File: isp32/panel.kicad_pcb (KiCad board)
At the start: 2 copper layers, 67 x 98 mm, 584 parts, among them J1 BAT1, J10 LoRa_ANT, J11 Power Modules, J12 Micro_SD_Card, J2 Switching, J3 USB_C_Receptacle_USB2.0, J4 ADC, J5 GPS_ANT, J6 F0, J7 F1, J8 BUZZ, J9 ANT, M1 Motor_Servo, M2 Motor_Servo, M3 Motor_Servo, M4 Motor_Servo, Q1 BSS138, Q2 S8050, Q3 IRLML6402, Q4 BSS138, Q5 IRLML6402, Q6 IRLML6402, Q8 BSS138, Q9 BSS138, SW1 RST, U1 AZ1117-3.3, U10 BMP280, U11 MPU-9250, U2 MP2315, U3 STM32G030F6, U4 AZ1117-1.8, U6 24LC32, U7 NEO-XM, U8 ESP32-S3-WROOM-1U, U9 RFM98W-315S2

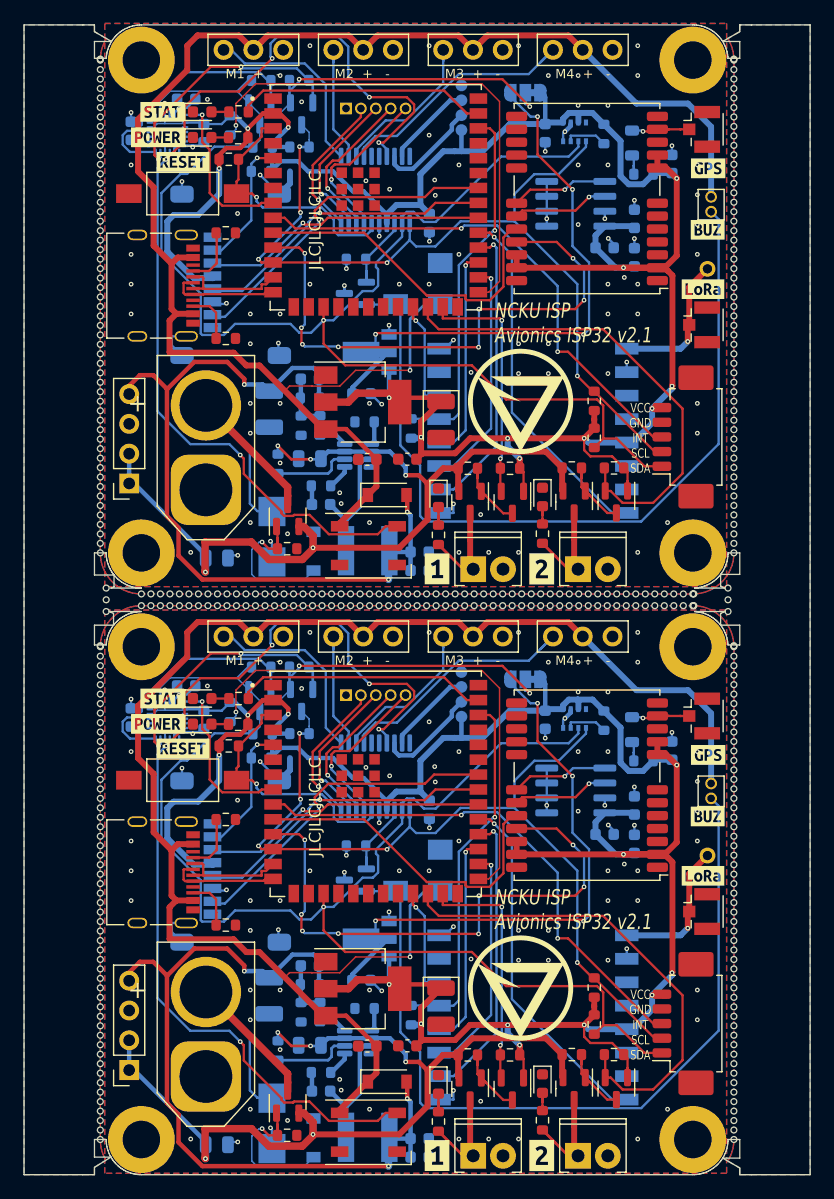
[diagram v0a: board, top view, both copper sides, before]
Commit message: chore: update isp32 project files
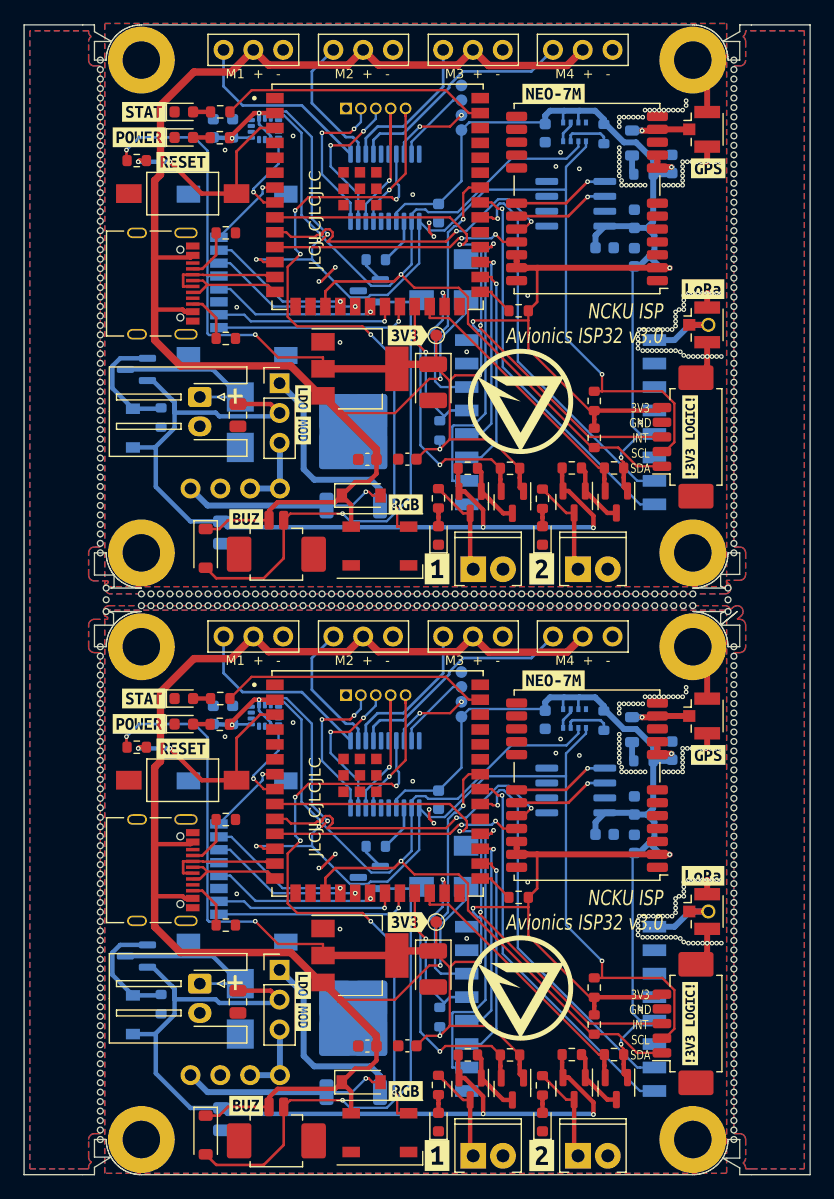
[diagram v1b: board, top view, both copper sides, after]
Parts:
- removed C1 (x2), C18 (x2), C8 (x2): 22u, Capacitor_SMD:C_0603_1608Metric
- removed the C12 at (107.0, 53.6)
- removed the C12 at (107.0, 103.6)
- removed the C15 at (87.9, 65.4)
- removed the C15 at (87.9, 115.4)
- removed C2 (x2): 220u, Capacitor_Tantalum_SMD:CP_EIA-3528-12_Kemet-T
- removed the C22 at (86.8, 29.2)
- removed the C22 at (86.8, 79.2)
- removed the C23 at (80.6, 79.0)
- removed the C23 at (80.6, 29.0)
- removed C24 (x2), C4 (x2): 100n, Capacitor_SMD:C_0603_1608Metric
- removed the C3 at (106.1, 86.9)
- removed the C3 at (106.1, 36.9)
- removed the C5 at (95.9, 107.0)
- removed the C5 at (95.9, 57.0)
- removed C7 (x2): NC, Capacitor_SMD:C_0603_1608Metric
- removed the D1 at (96.2, 114.9)
- removed the D1 at (96.2, 64.9)
- removed the D2 at (115.7, 110.2)
- removed the D2 at (115.7, 60.2)
- removed the D3 at (86.7, 77.4)
- removed the D3 at (86.7, 27.4)
- removed the D4 at (106.8, 60.3)
- removed the D4 at (106.8, 110.3)
- removed the D5 at (86.7, 29.6)
- removed the D5 at (86.7, 79.6)
- removed the D6 at (92.6, 113.6)
- removed the D6 at (92.6, 63.6)
- removed the D7 at (100.8, 114.4)
- removed the D7 at (100.8, 64.4)
- removed the D8 at (102.4, 110.1)
- removed the D8 at (102.4, 60.1)
- removed the J1 at (87.0, 109.6)
- removed the J1 at (87.0, 59.6)
- removed the J11 at (80.5, 59.1)
- removed the J11 at (80.5, 109.1)
- removed the J12 at (89.7, 91.3)
- removed the J12 at (89.7, 41.3)
- removed the J3 at (83.4, 42.2)
- removed the J3 at (83.4, 92.2)
- removed J8 (x2): BUZZ, Connector_PinHeader_1.27mm:PinHeader_1x02_P1.27mm_Vertical
- removed the J9 at (129.7, 90.8)
- removed the J9 at (129.7, 40.8)
- removed JP1 (x2): MPU VIO, Jumper:SolderJumper-3_P1.3mm_Bridged12_RoundedPad1.0x1.5mm_NumberLabels
- removed L3 (x2): 5.5, Inductor_SMD:L_Sunlord_SWPA5020S
- removed the LS1 at (105.1, 92.0)
- removed the LS1 at (105.1, 42.0)
- removed the Q2 at (99.7, 92.9)
- removed the Q2 at (99.7, 42.9)
- removed the Q6 at (94.0, 111.8)
- removed the Q6 at (94.0, 61.8)
- removed Q8 (x2), Q9 (x2): BSS138, Package_TO_SOT_SMD:SOT-23
- removed the R1 at (88.9, 31.5)
- removed the R1 at (88.9, 81.5)
- removed R10 (x2): 7k5, Resistor_SMD:R_0603_1608Metric
- removed R11 (x2): 40.2k, Resistor_SMD:R_0603_1608Metric
- removed R13 (x2), R17 (x2), R28 (x2), R29 (x2), R30 (x2), R33 (x2): 10k, Resistor_SMD:R_0603_1608Metric
- removed the R15 at (104.5, 54.4)
- removed the R15 at (104.5, 104.4)
- removed the R18 at (89.7, 29.6)
- removed the R18 at (89.7, 79.6)
- removed the R19 at (89.8, 77.4)
- removed the R19 at (89.8, 27.4)
- removed the R2 at (89.1, 28.6)
- removed the R2 at (89.1, 78.6)
- removed R21 (x2): 75k, Resistor_SMD:R_0603_1608Metric
- removed the R22 at (115.7, 113.4)
- removed the R22 at (115.7, 63.4)
- removed the R25 at (106.8, 63.5)
- removed the R25 at (106.8, 113.5)
- removed the R26 at (93.9, 64.6)
- removed the R26 at (93.9, 114.6)
- removed the R3 at (93.1, 57.4)
- removed the R3 at (93.1, 107.4)
- removed R8 (x2): 20, Resistor_SMD:R_0603_1608Metric
- removed R9 (x2): 20k, Resistor_SMD:R_0603_1608Metric
- removed REF** (x342): NPTH, NPTH
- removed the U1 at (100.4, 52.1)
- removed the U1 at (100.4, 102.1)
- removed U11 (x2): MPU-9250, Sensor_Motion:InvenSense_QFN-24_3x3mm_P0.4mm
- removed the U2 at (100.0, 106.7)
- removed the U2 at (100.0, 56.7)
- removed the U3 at (101.4, 84.1)
- removed the U3 at (101.4, 34.1)
- removed the U4 at (101.0, 47.9)
- removed the U4 at (101.0, 97.9)
- removed the U8 at (101.5, 34.7)
- removed the U8 at (101.5, 84.7)
- removed the U9 at (114.9, 54.6)
- removed the U9 at (114.9, 104.6)
- removed the kibuzzard-641A73E5 at (83.3, 27.4)
- removed the kibuzzard-641A73E5 at (83.3, 77.4)
- removed the kibuzzard-641A73FA at (82.9, 29.6)
- removed the kibuzzard-641A73FA at (82.9, 79.6)
- removed the kibuzzard-641A7704 at (129.8, 87.5)
- removed the kibuzzard-641A7704 at (129.8, 37.5)
- removed kibuzzard-642D96EE (x2): G***, kibuzzard-642D96EE
- removed kibuzzard-642D96F8 (x2): G***, kibuzzard-642D96F8
- removed the kibuzzard-642D97EE at (127.3, 104.1)
- removed the kibuzzard-642D97EE at (127.3, 54.1)
- added C12: 220u, Capacitor_Tantalum_SMD:CP_EIA-3528-12_Kemet-T, F.Cu at (106.4, 100.5)
- added C12: 220u, Capacitor_Tantalum_SMD:CP_EIA-3528-12_Kemet-T, F.Cu at (106.4, 50.5)
- added C15: 10u, Capacitor_SMD:C_0805_2012Metric, B.Cu at (88.3, 113.3)
- added C15: 10u, Capacitor_SMD:C_0805_2012Metric, B.Cu at (88.3, 63.3)
- added C22: 1u, Capacitor_SMD:C_0603_1608Metric, B.Cu at (87.6, 78.8)
- added C22: 1u, Capacitor_SMD:C_0603_1608Metric, B.Cu at (87.6, 28.8)
- added C23: 100n, Capacitor_SMD:C_0603_1608Metric, B.Cu at (89.3, 28.8)
- added C23: 100n, Capacitor_SMD:C_0603_1608Metric, B.Cu at (89.3, 78.8)
- added C3: 100n, Capacitor_SMD:C_0603_1608Metric, B.Cu at (106.8, 86.0)
- added C3: 100n, Capacitor_SMD:C_0603_1608Metric, B.Cu at (106.8, 36.0)
- added C5: 100n, Capacitor_SMD:C_0805_2012Metric, F.Cu at (89.7, 53.3)
- added C5: 100n, Capacitor_SMD:C_0805_2012Metric, F.Cu at (89.7, 103.3)
- added D1: Zener, Diode_SMD:D_SOD-123, B.Cu at (80.8, 54.4)
- added D1: Zener, Diode_SMD:D_SOD-123, B.Cu at (80.8, 104.4)
- added D2: F0_LED, LED_SMD:LED_0603_1608Metric, F.Cu at (115.7, 63.5)
- added D2: F0_LED, LED_SMD:LED_0603_1608Metric, F.Cu at (115.7, 113.5)
- added D3: ESP_LED, LED_SMD:LED_0603_1608Metric, F.Cu at (85.1, 77.4)
- added D3: ESP_LED, LED_SMD:LED_0603_1608Metric, F.Cu at (85.1, 27.4)
- added D4: F1_LED, LED_SMD:LED_0603_1608Metric, F.Cu at (106.8, 113.5)
- added D4: F1_LED, LED_SMD:LED_0603_1608Metric, F.Cu at (106.8, 63.5)
- added D5: POWER, LED_SMD:LED_0603_1608Metric, F.Cu at (85.1, 29.6)
- added D5: POWER, LED_SMD:LED_0603_1608Metric, F.Cu at (85.1, 79.6)
- added D6: TVS, Diode_SMD:D_SMB, B.Cu at (89.9, 103.9)
- added D6: TVS, Diode_SMD:D_SMB, B.Cu at (89.9, 53.9)
- added D7: WS2812B, LED_SMD:LED_WS2812B_PLCC4_5.0x5.0mm_P3.2mm, F.Cu at (101.8, 64.4)
- added D7: WS2812B, LED_SMD:LED_WS2812B_PLCC4_5.0x5.0mm_P3.2mm, F.Cu at (101.8, 114.4)
- added D8: D_Shockley, Diode_SMD:D_SOD-123, F.Cu at (100.2, 60.1)
- added D8: D_Shockley, Diode_SMD:D_SOD-123, F.Cu at (100.2, 110.1)
- added D9: D_Small, Diode_SMD:D_SOD-123, F.Cu at (87.0, 64.6)
- added D9: D_Small, Diode_SMD:D_SOD-123, F.Cu at (87.0, 114.6)
- added J1: BAT1, Connector_JST:JST_XH_S2B-XH-A-1_1x02_P2.50mm_Horizontal, F.Cu at (86.5, 101.7)
- added J1: BAT1, Connector_JST:JST_XH_S2B-XH-A-1_1x02_P2.50mm_Horizontal, F.Cu at (86.5, 51.7)
- added J11: Power Modules, Connector_PinSocket_2.54mm:PinSocket_1x04_P2.54mm_Vertical, B.Cu at (85.7, 59.5)
- added J11: Power Modules, Connector_PinSocket_2.54mm:PinSocket_1x04_P2.54mm_Vertical, B.Cu at (85.7, 109.5)
- added J12: Micro_SD_Card, Connector_Card:microSD_HC_Wuerth_693072010801, B.Cu at (89.7, 91.3)
- added J12: Micro_SD_Card, Connector_Card:microSD_HC_Wuerth_693072010801, B.Cu at (89.7, 41.3)
- added J13: VIN_SELECT, Connector_PinHeader_2.54mm:PinHeader_1x03_P2.54mm_Vertical, F.Cu at (93.3, 100.5)
- added J13: VIN_SELECT, Connector_PinHeader_2.54mm:PinHeader_1x03_P2.54mm_Vertical, F.Cu at (93.3, 50.5)
- added J14: BUZZ, Connector_Molex:Molex_PicoBlade_53261-0271_1x02-1MP_P1.25mm_Horizontal, F.Cu at (93.0, 64.6)
- added J14: BUZZ, Connector_Molex:Molex_PicoBlade_53261-0271_1x02-1MP_P1.25mm_Horizontal, F.Cu at (93.0, 114.6)
- added J3: USB_C_Receptacle_USB2.0, Connector_USB:USB_C_Receptacle_Palconn_UTC16-G, F.Cu at (83.4, 92.0)
- added J3: USB_C_Receptacle_USB2.0, Connector_USB:USB_C_Receptacle_Palconn_UTC16-G, F.Cu at (83.4, 42.0)
- added J9: ANT, Connector_PinHeader_2.00mm:PinHeader_1x01_P2.00mm_Vertical, B.Cu at (129.8, 95.6)
- added J9: ANT, Connector_PinHeader_2.00mm:PinHeader_1x01_P2.00mm_Vertical, B.Cu at (129.8, 45.6)
- added KiKit_MB_1_1: NPTH, NPTH, F.Cu at (78.0, 65.0)
- added KiKit_MB_1_10: NPTH, NPTH, F.Cu at (78.0, 57.7)
- added KiKit_MB_1_11: NPTH, NPTH, F.Cu at (78.0, 56.9)
- added KiKit_MB_1_12: NPTH, NPTH, F.Cu at (78.0, 56.1)
- added KiKit_MB_1_13: NPTH, NPTH, F.Cu at (78.0, 55.3)
- added KiKit_MB_1_14: NPTH, NPTH, F.Cu at (78.0, 54.5)
- added KiKit_MB_1_15: NPTH, NPTH, F.Cu at (78.0, 53.7)
- added KiKit_MB_1_16: NPTH, NPTH, F.Cu at (78.0, 52.9)
- added KiKit_MB_1_17: NPTH, NPTH, F.Cu at (78.0, 52.1)
- added KiKit_MB_1_18: NPTH, NPTH, F.Cu at (78.0, 51.3)
- added KiKit_MB_1_19: NPTH, NPTH, F.Cu at (78.0, 50.5)
- added KiKit_MB_1_2: NPTH, NPTH, F.Cu at (78.0, 64.2)
- added KiKit_MB_1_20: NPTH, NPTH, F.Cu at (78.0, 49.7)
- added KiKit_MB_1_21: NPTH, NPTH, F.Cu at (78.0, 48.8)
- added KiKit_MB_1_22: NPTH, NPTH, F.Cu at (78.0, 48.0)
- added KiKit_MB_1_23: NPTH, NPTH, F.Cu at (78.0, 47.2)
- added KiKit_MB_1_24: NPTH, NPTH, F.Cu at (78.0, 46.4)
- added KiKit_MB_1_25: NPTH, NPTH, F.Cu at (78.0, 45.6)
- added KiKit_MB_1_26: NPTH, NPTH, F.Cu at (78.0, 44.8)
- added KiKit_MB_1_27: NPTH, NPTH, F.Cu at (78.0, 44.0)
- added KiKit_MB_1_28: NPTH, NPTH, F.Cu at (78.0, 43.2)
- added KiKit_MB_1_29: NPTH, NPTH, F.Cu at (78.0, 42.4)
- added KiKit_MB_1_3: NPTH, NPTH, F.Cu at (78.0, 63.4)
- added KiKit_MB_1_30: NPTH, NPTH, F.Cu at (78.0, 41.6)
- added KiKit_MB_1_31: NPTH, NPTH, F.Cu at (78.0, 40.8)
- added KiKit_MB_1_32: NPTH, NPTH, F.Cu at (78.0, 40.0)
- added KiKit_MB_1_33: NPTH, NPTH, F.Cu at (78.0, 39.2)
- added KiKit_MB_1_34: NPTH, NPTH, F.Cu at (78.0, 38.3)
- added KiKit_MB_1_35: NPTH, NPTH, F.Cu at (78.0, 37.5)
- added KiKit_MB_1_36: NPTH, NPTH, F.Cu at (78.0, 36.7)
- added KiKit_MB_1_37: NPTH, NPTH, F.Cu at (78.0, 35.9)
- added KiKit_MB_1_38: NPTH, NPTH, F.Cu at (78.0, 35.1)
- added KiKit_MB_1_39: NPTH, NPTH, F.Cu at (78.0, 34.3)
- added KiKit_MB_1_4: NPTH, NPTH, F.Cu at (78.0, 62.6)
- added KiKit_MB_1_40: NPTH, NPTH, F.Cu at (78.0, 33.5)
- added KiKit_MB_1_41: NPTH, NPTH, F.Cu at (78.0, 32.7)
- added KiKit_MB_1_42: NPTH, NPTH, F.Cu at (78.0, 31.9)
- added KiKit_MB_1_43: NPTH, NPTH, F.Cu at (78.0, 31.1)
- added KiKit_MB_1_44: NPTH, NPTH, F.Cu at (78.0, 30.3)
- added KiKit_MB_1_45: NPTH, NPTH, F.Cu at (78.0, 29.5)
- added KiKit_MB_1_46: NPTH, NPTH, F.Cu at (78.0, 28.7)
- added KiKit_MB_1_47: NPTH, NPTH, F.Cu at (78.0, 27.8)
- added KiKit_MB_1_48: NPTH, NPTH, F.Cu at (78.0, 27.0)
- added KiKit_MB_1_49: NPTH, NPTH, F.Cu at (78.0, 26.2)
- added KiKit_MB_1_5: NPTH, NPTH, F.Cu at (78.0, 61.8)
- added KiKit_MB_1_50: NPTH, NPTH, F.Cu at (78.0, 25.4)
- added KiKit_MB_1_51: NPTH, NPTH, F.Cu at (78.0, 24.6)
- added KiKit_MB_1_52: NPTH, NPTH, F.Cu at (78.0, 23.8)
- added KiKit_MB_1_53: NPTH, NPTH, F.Cu at (78.0, 23.0)
- added KiKit_MB_1_6: NPTH, NPTH, F.Cu at (78.0, 61.0)
- added KiKit_MB_1_7: NPTH, NPTH, F.Cu at (78.0, 60.2)
- added KiKit_MB_1_8: NPTH, NPTH, F.Cu at (78.0, 59.3)
- added KiKit_MB_1_9: NPTH, NPTH, F.Cu at (78.0, 58.5)
- added KiKit_MB_2_1: NPTH, NPTH, F.Cu at (128.5, 68.5)
- added KiKit_MB_2_10: NPTH, NPTH, F.Cu at (121.2, 68.5)
- added KiKit_MB_2_11: NPTH, NPTH, F.Cu at (120.4, 68.5)
- added KiKit_MB_2_12: NPTH, NPTH, F.Cu at (119.6, 68.5)
- added KiKit_MB_2_13: NPTH, NPTH, F.Cu at (118.8, 68.5)
- added KiKit_MB_2_14: NPTH, NPTH, F.Cu at (118.0, 68.5)
- added KiKit_MB_2_15: NPTH, NPTH, F.Cu at (117.2, 68.5)
- added KiKit_MB_2_16: NPTH, NPTH, F.Cu at (116.3, 68.5)
- added KiKit_MB_2_17: NPTH, NPTH, F.Cu at (115.5, 68.5)
- added KiKit_MB_2_18: NPTH, NPTH, F.Cu at (114.7, 68.5)
- added KiKit_MB_2_19: NPTH, NPTH, F.Cu at (113.9, 68.5)
- added KiKit_MB_2_2: NPTH, NPTH, F.Cu at (127.7, 68.5)
- added KiKit_MB_2_20: NPTH, NPTH, F.Cu at (113.1, 68.5)
- added KiKit_MB_2_21: NPTH, NPTH, F.Cu at (112.3, 68.5)
- added KiKit_MB_2_22: NPTH, NPTH, F.Cu at (111.5, 68.5)
- added KiKit_MB_2_23: NPTH, NPTH, F.Cu at (110.7, 68.5)
- added KiKit_MB_2_24: NPTH, NPTH, F.Cu at (109.9, 68.5)
- added KiKit_MB_2_25: NPTH, NPTH, F.Cu at (109.1, 68.5)
- added KiKit_MB_2_26: NPTH, NPTH, F.Cu at (108.2, 68.5)
- added KiKit_MB_2_27: NPTH, NPTH, F.Cu at (107.4, 68.5)
- added KiKit_MB_2_28: NPTH, NPTH, F.Cu at (106.6, 68.5)
- added KiKit_MB_2_29: NPTH, NPTH, F.Cu at (105.8, 68.5)
- added KiKit_MB_2_3: NPTH, NPTH, F.Cu at (126.9, 68.5)
- added KiKit_MB_2_30: NPTH, NPTH, F.Cu at (105.0, 68.5)
- added KiKit_MB_2_31: NPTH, NPTH, F.Cu at (104.2, 68.5)
- added KiKit_MB_2_32: NPTH, NPTH, F.Cu at (103.4, 68.5)
- added KiKit_MB_2_33: NPTH, NPTH, F.Cu at (102.6, 68.5)
- added KiKit_MB_2_34: NPTH, NPTH, F.Cu at (101.8, 68.5)
- added KiKit_MB_2_35: NPTH, NPTH, F.Cu at (100.9, 68.5)
- added KiKit_MB_2_36: NPTH, NPTH, F.Cu at (100.1, 68.5)
- added KiKit_MB_2_37: NPTH, NPTH, F.Cu at (99.3, 68.5)
- added KiKit_MB_2_38: NPTH, NPTH, F.Cu at (98.5, 68.5)
- added KiKit_MB_2_39: NPTH, NPTH, F.Cu at (97.7, 68.5)
- added KiKit_MB_2_4: NPTH, NPTH, F.Cu at (126.1, 68.5)
- added KiKit_MB_2_40: NPTH, NPTH, F.Cu at (96.9, 68.5)
- added KiKit_MB_2_41: NPTH, NPTH, F.Cu at (96.1, 68.5)
- added KiKit_MB_2_42: NPTH, NPTH, F.Cu at (95.3, 68.5)
- added KiKit_MB_2_43: NPTH, NPTH, F.Cu at (94.5, 68.5)
- added KiKit_MB_2_44: NPTH, NPTH, F.Cu at (93.7, 68.5)
- added KiKit_MB_2_45: NPTH, NPTH, F.Cu at (92.8, 68.5)
- added KiKit_MB_2_46: NPTH, NPTH, F.Cu at (92.0, 68.5)
- added KiKit_MB_2_47: NPTH, NPTH, F.Cu at (91.2, 68.5)
- added KiKit_MB_2_48: NPTH, NPTH, F.Cu at (90.4, 68.5)
- added KiKit_MB_2_49: NPTH, NPTH, F.Cu at (89.6, 68.5)
- added KiKit_MB_2_5: NPTH, NPTH, F.Cu at (125.3, 68.5)
- added KiKit_MB_2_50: NPTH, NPTH, F.Cu at (88.8, 68.5)
- added KiKit_MB_2_51: NPTH, NPTH, F.Cu at (88.0, 68.5)
- added KiKit_MB_2_52: NPTH, NPTH, F.Cu at (87.2, 68.5)
- added KiKit_MB_2_53: NPTH, NPTH, F.Cu at (86.4, 68.5)
- added KiKit_MB_2_54: NPTH, NPTH, F.Cu at (85.6, 68.5)
- added KiKit_MB_2_55: NPTH, NPTH, F.Cu at (84.7, 68.5)
- added KiKit_MB_2_56: NPTH, NPTH, F.Cu at (83.9, 68.5)
- added KiKit_MB_2_57: NPTH, NPTH, F.Cu at (83.1, 68.5)
- added KiKit_MB_2_58: NPTH, NPTH, F.Cu at (82.3, 68.5)
- added KiKit_MB_2_59: NPTH, NPTH, F.Cu at (81.5, 68.5)
- added KiKit_MB_2_6: NPTH, NPTH, F.Cu at (124.4, 68.5)
- added KiKit_MB_2_7: NPTH, NPTH, F.Cu at (123.6, 68.5)
- added KiKit_MB_2_8: NPTH, NPTH, F.Cu at (122.8, 68.5)
- added KiKit_MB_2_9: NPTH, NPTH, F.Cu at (122.0, 68.5)
- added KiKit_MB_3_1: NPTH, NPTH, F.Cu at (132.0, 23.0)
- added KiKit_MB_3_10: NPTH, NPTH, F.Cu at (132.0, 30.3)
- added KiKit_MB_3_11: NPTH, NPTH, F.Cu at (132.0, 31.1)
- added KiKit_MB_3_12: NPTH, NPTH, F.Cu at (132.0, 31.9)
- added KiKit_MB_3_13: NPTH, NPTH, F.Cu at (132.0, 32.7)
- added KiKit_MB_3_14: NPTH, NPTH, F.Cu at (132.0, 33.5)
- added KiKit_MB_3_15: NPTH, NPTH, F.Cu at (132.0, 34.3)
- added KiKit_MB_3_16: NPTH, NPTH, F.Cu at (132.0, 35.1)
- added KiKit_MB_3_17: NPTH, NPTH, F.Cu at (132.0, 35.9)
- added KiKit_MB_3_18: NPTH, NPTH, F.Cu at (132.0, 36.7)
- added KiKit_MB_3_19: NPTH, NPTH, F.Cu at (132.0, 37.5)
- added KiKit_MB_3_2: NPTH, NPTH, F.Cu at (132.0, 23.8)
- added KiKit_MB_3_20: NPTH, NPTH, F.Cu at (132.0, 38.3)
- added KiKit_MB_3_21: NPTH, NPTH, F.Cu at (132.0, 39.2)
- added KiKit_MB_3_22: NPTH, NPTH, F.Cu at (132.0, 40.0)
- added KiKit_MB_3_23: NPTH, NPTH, F.Cu at (132.0, 40.8)
- added KiKit_MB_3_24: NPTH, NPTH, F.Cu at (132.0, 41.6)
- added KiKit_MB_3_25: NPTH, NPTH, F.Cu at (132.0, 42.4)
- added KiKit_MB_3_26: NPTH, NPTH, F.Cu at (132.0, 43.2)
- added KiKit_MB_3_27: NPTH, NPTH, F.Cu at (132.0, 44.0)
- added KiKit_MB_3_28: NPTH, NPTH, F.Cu at (132.0, 44.8)
- added KiKit_MB_3_29: NPTH, NPTH, F.Cu at (132.0, 45.6)
- added KiKit_MB_3_3: NPTH, NPTH, F.Cu at (132.0, 24.6)
- added KiKit_MB_3_30: NPTH, NPTH, F.Cu at (132.0, 46.4)
- added KiKit_MB_3_31: NPTH, NPTH, F.Cu at (132.0, 47.2)
- added KiKit_MB_3_32: NPTH, NPTH, F.Cu at (132.0, 48.0)
- added KiKit_MB_3_33: NPTH, NPTH, F.Cu at (132.0, 48.8)
- added KiKit_MB_3_34: NPTH, NPTH, F.Cu at (132.0, 49.7)
- added KiKit_MB_3_35: NPTH, NPTH, F.Cu at (132.0, 50.5)
- added KiKit_MB_3_36: NPTH, NPTH, F.Cu at (132.0, 51.3)
- added KiKit_MB_3_37: NPTH, NPTH, F.Cu at (132.0, 52.1)
- added KiKit_MB_3_38: NPTH, NPTH, F.Cu at (132.0, 52.9)
- added KiKit_MB_3_39: NPTH, NPTH, F.Cu at (132.0, 53.7)
- added KiKit_MB_3_4: NPTH, NPTH, F.Cu at (132.0, 25.4)
- added KiKit_MB_3_40: NPTH, NPTH, F.Cu at (132.0, 54.5)
- added KiKit_MB_3_41: NPTH, NPTH, F.Cu at (132.0, 55.3)
- added KiKit_MB_3_42: NPTH, NPTH, F.Cu at (132.0, 56.1)
- added KiKit_MB_3_43: NPTH, NPTH, F.Cu at (132.0, 56.9)
- added KiKit_MB_3_44: NPTH, NPTH, F.Cu at (132.0, 57.7)
- added KiKit_MB_3_45: NPTH, NPTH, F.Cu at (132.0, 58.5)
- added KiKit_MB_3_46: NPTH, NPTH, F.Cu at (132.0, 59.3)
- added KiKit_MB_3_47: NPTH, NPTH, F.Cu at (132.0, 60.2)
- added KiKit_MB_3_48: NPTH, NPTH, F.Cu at (132.0, 61.0)
- added KiKit_MB_3_49: NPTH, NPTH, F.Cu at (132.0, 61.8)
- added KiKit_MB_3_5: NPTH, NPTH, F.Cu at (132.0, 26.2)
- added KiKit_MB_3_50: NPTH, NPTH, F.Cu at (132.0, 62.6)
- added KiKit_MB_3_51: NPTH, NPTH, F.Cu at (132.0, 63.4)
- added KiKit_MB_3_52: NPTH, NPTH, F.Cu at (132.0, 64.2)
- added KiKit_MB_3_53: NPTH, NPTH, F.Cu at (132.0, 65.0)
- added KiKit_MB_3_6: NPTH, NPTH, F.Cu at (132.0, 27.0)
- added KiKit_MB_3_7: NPTH, NPTH, F.Cu at (132.0, 27.8)
- added KiKit_MB_3_8: NPTH, NPTH, F.Cu at (132.0, 28.7)
- added KiKit_MB_3_9: NPTH, NPTH, F.Cu at (132.0, 29.5)
- added KiKit_MB_4_1: NPTH, NPTH, F.Cu at (78.0, 115.0)
- added KiKit_MB_4_10: NPTH, NPTH, F.Cu at (78.0, 107.7)
- added KiKit_MB_4_11: NPTH, NPTH, F.Cu at (78.0, 106.9)
- added KiKit_MB_4_12: NPTH, NPTH, F.Cu at (78.0, 106.1)
- added KiKit_MB_4_13: NPTH, NPTH, F.Cu at (78.0, 105.3)
- added KiKit_MB_4_14: NPTH, NPTH, F.Cu at (78.0, 104.5)
- added KiKit_MB_4_15: NPTH, NPTH, F.Cu at (78.0, 103.7)
- added KiKit_MB_4_16: NPTH, NPTH, F.Cu at (78.0, 102.9)
- added KiKit_MB_4_17: NPTH, NPTH, F.Cu at (78.0, 102.1)
- added KiKit_MB_4_18: NPTH, NPTH, F.Cu at (78.0, 101.3)
- added KiKit_MB_4_19: NPTH, NPTH, F.Cu at (78.0, 100.5)
- added KiKit_MB_4_2: NPTH, NPTH, F.Cu at (78.0, 114.2)
- added KiKit_MB_4_20: NPTH, NPTH, F.Cu at (78.0, 99.7)
- added KiKit_MB_4_21: NPTH, NPTH, F.Cu at (78.0, 98.8)
- added KiKit_MB_4_22: NPTH, NPTH, F.Cu at (78.0, 98.0)
- added KiKit_MB_4_23: NPTH, NPTH, F.Cu at (78.0, 97.2)
- added KiKit_MB_4_24: NPTH, NPTH, F.Cu at (78.0, 96.4)
- added KiKit_MB_4_25: NPTH, NPTH, F.Cu at (78.0, 95.6)
- added KiKit_MB_4_26: NPTH, NPTH, F.Cu at (78.0, 94.8)
- added KiKit_MB_4_27: NPTH, NPTH, F.Cu at (78.0, 94.0)
- added KiKit_MB_4_28: NPTH, NPTH, F.Cu at (78.0, 93.2)
- added KiKit_MB_4_29: NPTH, NPTH, F.Cu at (78.0, 92.4)
- added KiKit_MB_4_3: NPTH, NPTH, F.Cu at (78.0, 113.4)
- added KiKit_MB_4_30: NPTH, NPTH, F.Cu at (78.0, 91.6)
- added KiKit_MB_4_31: NPTH, NPTH, F.Cu at (78.0, 90.8)
- added KiKit_MB_4_32: NPTH, NPTH, F.Cu at (78.0, 90.0)
- added KiKit_MB_4_33: NPTH, NPTH, F.Cu at (78.0, 89.2)
- added KiKit_MB_4_34: NPTH, NPTH, F.Cu at (78.0, 88.3)
- added KiKit_MB_4_35: NPTH, NPTH, F.Cu at (78.0, 87.5)
- added KiKit_MB_4_36: NPTH, NPTH, F.Cu at (78.0, 86.7)
- added KiKit_MB_4_37: NPTH, NPTH, F.Cu at (78.0, 85.9)
- added KiKit_MB_4_38: NPTH, NPTH, F.Cu at (78.0, 85.1)
- added KiKit_MB_4_39: NPTH, NPTH, F.Cu at (78.0, 84.3)
- added KiKit_MB_4_4: NPTH, NPTH, F.Cu at (78.0, 112.6)
- added KiKit_MB_4_40: NPTH, NPTH, F.Cu at (78.0, 83.5)
- added KiKit_MB_4_41: NPTH, NPTH, F.Cu at (78.0, 82.7)
- added KiKit_MB_4_42: NPTH, NPTH, F.Cu at (78.0, 81.9)
- added KiKit_MB_4_43: NPTH, NPTH, F.Cu at (78.0, 81.1)
- added KiKit_MB_4_44: NPTH, NPTH, F.Cu at (78.0, 80.3)
- added KiKit_MB_4_45: NPTH, NPTH, F.Cu at (78.0, 79.5)
- added KiKit_MB_4_46: NPTH, NPTH, F.Cu at (78.0, 78.7)
- added KiKit_MB_4_47: NPTH, NPTH, F.Cu at (78.0, 77.8)
- added KiKit_MB_4_48: NPTH, NPTH, F.Cu at (78.0, 77.0)
- added KiKit_MB_4_49: NPTH, NPTH, F.Cu at (78.0, 76.2)
- added KiKit_MB_4_5: NPTH, NPTH, F.Cu at (78.0, 111.8)
- added KiKit_MB_4_50: NPTH, NPTH, F.Cu at (78.0, 75.4)
- added KiKit_MB_4_51: NPTH, NPTH, F.Cu at (78.0, 74.6)
- added KiKit_MB_4_52: NPTH, NPTH, F.Cu at (78.0, 73.8)
- added KiKit_MB_4_53: NPTH, NPTH, F.Cu at (78.0, 73.0)
- added KiKit_MB_4_6: NPTH, NPTH, F.Cu at (78.0, 111.0)
- added KiKit_MB_4_7: NPTH, NPTH, F.Cu at (78.0, 110.2)
- added KiKit_MB_4_8: NPTH, NPTH, F.Cu at (78.0, 109.3)
- added KiKit_MB_4_9: NPTH, NPTH, F.Cu at (78.0, 108.5)
- added KiKit_MB_5_1: NPTH, NPTH, F.Cu at (81.5, 69.5)
- added KiKit_MB_5_10: NPTH, NPTH, F.Cu at (88.8, 69.5)
- added KiKit_MB_5_11: NPTH, NPTH, F.Cu at (89.6, 69.5)
- added KiKit_MB_5_12: NPTH, NPTH, F.Cu at (90.4, 69.5)
- added KiKit_MB_5_13: NPTH, NPTH, F.Cu at (91.2, 69.5)
- added KiKit_MB_5_14: NPTH, NPTH, F.Cu at (92.0, 69.5)
- added KiKit_MB_5_15: NPTH, NPTH, F.Cu at (92.8, 69.5)
- added KiKit_MB_5_16: NPTH, NPTH, F.Cu at (93.7, 69.5)
- added KiKit_MB_5_17: NPTH, NPTH, F.Cu at (94.5, 69.5)
- added KiKit_MB_5_18: NPTH, NPTH, F.Cu at (95.3, 69.5)
- added KiKit_MB_5_19: NPTH, NPTH, F.Cu at (96.1, 69.5)
- added KiKit_MB_5_2: NPTH, NPTH, F.Cu at (82.3, 69.5)
- added KiKit_MB_5_20: NPTH, NPTH, F.Cu at (96.9, 69.5)
- added KiKit_MB_5_21: NPTH, NPTH, F.Cu at (97.7, 69.5)
- added KiKit_MB_5_22: NPTH, NPTH, F.Cu at (98.5, 69.5)
- added KiKit_MB_5_23: NPTH, NPTH, F.Cu at (99.3, 69.5)
- added KiKit_MB_5_24: NPTH, NPTH, F.Cu at (100.1, 69.5)
- added KiKit_MB_5_25: NPTH, NPTH, F.Cu at (100.9, 69.5)
- added KiKit_MB_5_26: NPTH, NPTH, F.Cu at (101.8, 69.5)
- added KiKit_MB_5_27: NPTH, NPTH, F.Cu at (102.6, 69.5)
- added KiKit_MB_5_28: NPTH, NPTH, F.Cu at (103.4, 69.5)
- added KiKit_MB_5_29: NPTH, NPTH, F.Cu at (104.2, 69.5)
- added KiKit_MB_5_3: NPTH, NPTH, F.Cu at (83.1, 69.5)
- added KiKit_MB_5_30: NPTH, NPTH, F.Cu at (105.0, 69.5)
- added KiKit_MB_5_31: NPTH, NPTH, F.Cu at (105.8, 69.5)
- added KiKit_MB_5_32: NPTH, NPTH, F.Cu at (106.6, 69.5)
- added KiKit_MB_5_33: NPTH, NPTH, F.Cu at (107.4, 69.5)
- added KiKit_MB_5_34: NPTH, NPTH, F.Cu at (108.2, 69.5)
- added KiKit_MB_5_35: NPTH, NPTH, F.Cu at (109.1, 69.5)
- added KiKit_MB_5_36: NPTH, NPTH, F.Cu at (109.9, 69.5)
- added KiKit_MB_5_37: NPTH, NPTH, F.Cu at (110.7, 69.5)
- added KiKit_MB_5_38: NPTH, NPTH, F.Cu at (111.5, 69.5)
- added KiKit_MB_5_39: NPTH, NPTH, F.Cu at (112.3, 69.5)
- added KiKit_MB_5_4: NPTH, NPTH, F.Cu at (83.9, 69.5)
- added KiKit_MB_5_40: NPTH, NPTH, F.Cu at (113.1, 69.5)
- added KiKit_MB_5_41: NPTH, NPTH, F.Cu at (113.9, 69.5)
- added KiKit_MB_5_42: NPTH, NPTH, F.Cu at (114.7, 69.5)
- added KiKit_MB_5_43: NPTH, NPTH, F.Cu at (115.5, 69.5)
- added KiKit_MB_5_44: NPTH, NPTH, F.Cu at (116.3, 69.5)
- added KiKit_MB_5_45: NPTH, NPTH, F.Cu at (117.2, 69.5)
- added KiKit_MB_5_46: NPTH, NPTH, F.Cu at (118.0, 69.5)
- added KiKit_MB_5_47: NPTH, NPTH, F.Cu at (118.8, 69.5)
- added KiKit_MB_5_48: NPTH, NPTH, F.Cu at (119.6, 69.5)
- added KiKit_MB_5_49: NPTH, NPTH, F.Cu at (120.4, 69.5)
- added KiKit_MB_5_5: NPTH, NPTH, F.Cu at (84.7, 69.5)
- added KiKit_MB_5_50: NPTH, NPTH, F.Cu at (121.2, 69.5)
- added KiKit_MB_5_51: NPTH, NPTH, F.Cu at (122.0, 69.5)
- added KiKit_MB_5_52: NPTH, NPTH, F.Cu at (122.8, 69.5)
- added KiKit_MB_5_53: NPTH, NPTH, F.Cu at (123.6, 69.5)
- added KiKit_MB_5_54: NPTH, NPTH, F.Cu at (124.4, 69.5)
- added KiKit_MB_5_55: NPTH, NPTH, F.Cu at (125.3, 69.5)
- added KiKit_MB_5_56: NPTH, NPTH, F.Cu at (126.1, 69.5)
- added KiKit_MB_5_57: NPTH, NPTH, F.Cu at (126.9, 69.5)
- added KiKit_MB_5_58: NPTH, NPTH, F.Cu at (127.7, 69.5)
- added KiKit_MB_5_59: NPTH, NPTH, F.Cu at (128.5, 69.5)
- added KiKit_MB_5_6: NPTH, NPTH, F.Cu at (85.6, 69.5)
- added KiKit_MB_5_7: NPTH, NPTH, F.Cu at (86.4, 69.5)
- added KiKit_MB_5_8: NPTH, NPTH, F.Cu at (87.2, 69.5)
- added KiKit_MB_5_9: NPTH, NPTH, F.Cu at (88.0, 69.5)
- added KiKit_MB_6_1: NPTH, NPTH, F.Cu at (132.0, 73.0)
- added KiKit_MB_6_10: NPTH, NPTH, F.Cu at (132.0, 80.3)
- added KiKit_MB_6_11: NPTH, NPTH, F.Cu at (132.0, 81.1)
- added KiKit_MB_6_12: NPTH, NPTH, F.Cu at (132.0, 81.9)
- added KiKit_MB_6_13: NPTH, NPTH, F.Cu at (132.0, 82.7)
- added KiKit_MB_6_14: NPTH, NPTH, F.Cu at (132.0, 83.5)
- added KiKit_MB_6_15: NPTH, NPTH, F.Cu at (132.0, 84.3)
- added KiKit_MB_6_16: NPTH, NPTH, F.Cu at (132.0, 85.1)
- added KiKit_MB_6_17: NPTH, NPTH, F.Cu at (132.0, 85.9)
- added KiKit_MB_6_18: NPTH, NPTH, F.Cu at (132.0, 86.7)
- added KiKit_MB_6_19: NPTH, NPTH, F.Cu at (132.0, 87.5)
- added KiKit_MB_6_2: NPTH, NPTH, F.Cu at (132.0, 73.8)
- added KiKit_MB_6_20: NPTH, NPTH, F.Cu at (132.0, 88.3)
- added KiKit_MB_6_21: NPTH, NPTH, F.Cu at (132.0, 89.2)
- added KiKit_MB_6_22: NPTH, NPTH, F.Cu at (132.0, 90.0)
- added KiKit_MB_6_23: NPTH, NPTH, F.Cu at (132.0, 90.8)
- added KiKit_MB_6_24: NPTH, NPTH, F.Cu at (132.0, 91.6)
- added KiKit_MB_6_25: NPTH, NPTH, F.Cu at (132.0, 92.4)
- added KiKit_MB_6_26: NPTH, NPTH, F.Cu at (132.0, 93.2)
- added KiKit_MB_6_27: NPTH, NPTH, F.Cu at (132.0, 94.0)
- added KiKit_MB_6_28: NPTH, NPTH, F.Cu at (132.0, 94.8)
- added KiKit_MB_6_29: NPTH, NPTH, F.Cu at (132.0, 95.6)
- added KiKit_MB_6_3: NPTH, NPTH, F.Cu at (132.0, 74.6)
- added KiKit_MB_6_30: NPTH, NPTH, F.Cu at (132.0, 96.4)
- added KiKit_MB_6_31: NPTH, NPTH, F.Cu at (132.0, 97.2)
- added KiKit_MB_6_32: NPTH, NPTH, F.Cu at (132.0, 98.0)
- added KiKit_MB_6_33: NPTH, NPTH, F.Cu at (132.0, 98.8)
- added KiKit_MB_6_34: NPTH, NPTH, F.Cu at (132.0, 99.7)
- added KiKit_MB_6_35: NPTH, NPTH, F.Cu at (132.0, 100.5)
- added KiKit_MB_6_36: NPTH, NPTH, F.Cu at (132.0, 101.3)
- added KiKit_MB_6_37: NPTH, NPTH, F.Cu at (132.0, 102.1)
- added KiKit_MB_6_38: NPTH, NPTH, F.Cu at (132.0, 102.9)
- added KiKit_MB_6_39: NPTH, NPTH, F.Cu at (132.0, 103.7)
- added KiKit_MB_6_4: NPTH, NPTH, F.Cu at (132.0, 75.4)
- added KiKit_MB_6_40: NPTH, NPTH, F.Cu at (132.0, 104.5)
- added KiKit_MB_6_41: NPTH, NPTH, F.Cu at (132.0, 105.3)
- added KiKit_MB_6_42: NPTH, NPTH, F.Cu at (132.0, 106.1)
- added KiKit_MB_6_43: NPTH, NPTH, F.Cu at (132.0, 106.9)
- added KiKit_MB_6_44: NPTH, NPTH, F.Cu at (132.0, 107.7)
- added KiKit_MB_6_45: NPTH, NPTH, F.Cu at (132.0, 108.5)
- added KiKit_MB_6_46: NPTH, NPTH, F.Cu at (132.0, 109.3)
- added KiKit_MB_6_47: NPTH, NPTH, F.Cu at (132.0, 110.2)
- added KiKit_MB_6_48: NPTH, NPTH, F.Cu at (132.0, 111.0)
- added KiKit_MB_6_49: NPTH, NPTH, F.Cu at (132.0, 111.8)
- added KiKit_MB_6_5: NPTH, NPTH, F.Cu at (132.0, 76.2)
- added KiKit_MB_6_50: NPTH, NPTH, F.Cu at (132.0, 112.6)
- added KiKit_MB_6_51: NPTH, NPTH, F.Cu at (132.0, 113.4)
- added KiKit_MB_6_52: NPTH, NPTH, F.Cu at (132.0, 114.2)
- added KiKit_MB_6_53: NPTH, NPTH, F.Cu at (132.0, 115.0)
- added KiKit_MB_6_6: NPTH, NPTH, F.Cu at (132.0, 77.0)
- added KiKit_MB_6_7: NPTH, NPTH, F.Cu at (132.0, 77.8)
- added KiKit_MB_6_8: NPTH, NPTH, F.Cu at (132.0, 78.7)
- added KiKit_MB_6_9: NPTH, NPTH, F.Cu at (132.0, 79.5)
- added KiKit_MB_7_1: NPTH, NPTH, F.Cu at (78.5, 68.0)
- added KiKit_MB_7_2: NPTH, NPTH, F.Cu at (78.5, 69.0)
- added KiKit_MB_7_3: NPTH, NPTH, F.Cu at (78.5, 70.0)
- added KiKit_MB_8_1: NPTH, NPTH, F.Cu at (131.5, 68.0)
- added KiKit_MB_8_2: NPTH, NPTH, F.Cu at (131.5, 69.0)
- added KiKit_MB_8_3: NPTH, NPTH, F.Cu at (131.5, 70.0)
- added LS1: 5020, Buzzer:XDCR_KSSG33J12-3, B.Cu at (107.3, 91.7)
- added LS1: 5020, Buzzer:XDCR_KSSG33J12-3, B.Cu at (107.3, 41.7)
- added Q2: S8050, Package_TO_SOT_SMD:SOT-23, B.Cu at (100.9, 92.7)
- added Q2: S8050, Package_TO_SOT_SMD:SOT-23, B.Cu at (100.9, 42.7)
- added Q6: IRLML6402, Package_TO_SOT_SMD:SOT-23, B.Cu at (81.1, 99.4)
- added Q6: IRLML6402, Package_TO_SOT_SMD:SOT-23, B.Cu at (81.1, 49.4)
- added R1: 10k, Resistor_SMD:R_0603_1608Metric, F.Cu at (81.1, 31.6)
- added R1: 10k, Resistor_SMD:R_0603_1608Metric, F.Cu at (81.1, 81.6)
- added R15: 10k, Resistor_SMD:R_0603_1608Metric, B.Cu at (106.9, 54.6)
- added R15: 10k, Resistor_SMD:R_0603_1608Metric, B.Cu at (106.9, 104.6)
- added R18: 1k, Resistor_SMD:R_0603_1608Metric, F.Cu at (88.2, 79.6)
- added R18: 1k, Resistor_SMD:R_0603_1608Metric, F.Cu at (88.2, 29.6)
- added R19: 1k, Resistor_SMD:R_0603_1608Metric, F.Cu at (88.2, 27.4)
- added R19: 1k, Resistor_SMD:R_0603_1608Metric, F.Cu at (88.2, 77.4)
- added R2: 10k, Resistor_SMD:R_0603_1608Metric, F.Cu at (113.7, 94.4)
- added R2: 10k, Resistor_SMD:R_0603_1608Metric, F.Cu at (113.7, 44.4)
- added R22: 10k, Resistor_SMD:R_0603_1608Metric, F.Cu at (115.7, 110.4)
- added R22: 10k, Resistor_SMD:R_0603_1608Metric, F.Cu at (115.7, 60.4)
- added R25: 10k, Resistor_SMD:R_0603_1608Metric, F.Cu at (106.8, 110.4)
- added R25: 10k, Resistor_SMD:R_0603_1608Metric, F.Cu at (106.8, 60.4)
- added R26: 100k, Resistor_SMD:R_0603_1608Metric, B.Cu at (83.2, 53.5)
- added R26: 100k, Resistor_SMD:R_0603_1608Metric, B.Cu at (83.2, 103.5)
- added R3: 100, Resistor_SMD:R_0603_1608Metric, B.Cu at (101.5, 90.0)
- added R3: 100, Resistor_SMD:R_0603_1608Metric, B.Cu at (101.5, 40.0)
- added TP2: TP-3V3, TestPoint:TestPoint_Pad_D1.0mm, F.Cu at (106.6, 96.5)
- added TP2: TP-3V3, TestPoint:TestPoint_Pad_D1.0mm, F.Cu at (106.6, 46.5)
- added U1: AZ1117-3.3, Package_TO_SOT_SMD:SOT-223-3_TabPin2, F.Cu at (100.1, 99.3)
- added U1: AZ1117-3.3, Package_TO_SOT_SMD:SOT-223-3_TabPin2, F.Cu at (100.1, 49.3)
- added U2: BA05C, Package_TO_SOT_SMD:TO-252-2, B.Cu at (99.6, 105.9)
- added U2: BA05C, Package_TO_SOT_SMD:TO-252-2, B.Cu at (99.6, 55.9)
- added U3: STM32G030F6, Package_SO:TSSOP-20_4.4x6.5mm_P0.65mm, B.Cu at (102.3, 83.9)
- added U3: STM32G030F6, Package_SO:TSSOP-20_4.4x6.5mm_P0.65mm, B.Cu at (102.3, 33.9)
- added U4: LSM6DSM, Package_LGA:LGA-14_3x2.5mm_P0.5mm_LayoutBorder3x4y, B.Cu at (92.0, 78.9)
- added U4: LSM6DSM, Package_LGA:LGA-14_3x2.5mm_P0.5mm_LayoutBorder3x4y, B.Cu at (92.0, 28.9)
- added U8: ESP32-S3-WROOM-1U, ESP32-S3-WROOM-1U:XCVR_ESP32-S3-WROOM-1U, F.Cu at (101.6, 34.7)
- added U8: ESP32-S3-WROOM-1U, ESP32-S3-WROOM-1U:XCVR_ESP32-S3-WROOM-1U, F.Cu at (101.6, 84.7)
- added U9: RFM98W-315S2, RF_Module:HOPERF_RFM9XW_SMD, B.Cu at (117.2, 103.9)
- added U9: RFM98W-315S2, RF_Module:HOPERF_RFM9XW_SMD, B.Cu at (117.2, 53.9)
- added kibuzzard-641A73E5: G***, kibuzzard-641A73E5, F.Cu at (81.7, 27.4)
- added kibuzzard-641A73E5: G***, kibuzzard-641A73E5, F.Cu at (81.7, 77.4)
- added kibuzzard-641A73FA: G***, kibuzzard-641A73FA, F.Cu at (81.3, 29.6)
- added kibuzzard-641A73FA: G***, kibuzzard-641A73FA, F.Cu at (81.3, 79.6)
- added kibuzzard-641A7704: G***, kibuzzard-641A7704, F.Cu at (90.4, 112.1)
- added kibuzzard-641A7704: G***, kibuzzard-641A7704, F.Cu at (90.4, 62.1)
- added kibuzzard-642D97EE: G***, kibuzzard-642D97EE, B.Cu at (128.9, 105.1)
- added kibuzzard-642D97EE: G***, kibuzzard-642D97EE, B.Cu at (128.9, 55.1)
- added kibuzzard-661FABB5: G***, kibuzzard-661FABB5, B.Cu at (118.5, 76.8)
- added kibuzzard-661FABB5: G***, kibuzzard-661FABB5, B.Cu at (118.5, 26.8)
- added kibuzzard-661FAECF: G***, kibuzzard-661FAECF, F.Cu at (128.3, 55.1)
- added kibuzzard-661FAECF: G***, kibuzzard-661FAECF, F.Cu at (128.3, 105.1)
- added kibuzzard-661FBC0A: G***, kibuzzard-661FBC0A, F.Cu at (95.3, 54.6)
- added kibuzzard-661FBC0A: G***, kibuzzard-661FBC0A, F.Cu at (95.3, 104.6)
- added kibuzzard-661FBC21: G***, kibuzzard-661FBC21, F.Cu at (95.3, 101.9)
- added kibuzzard-661FBC21: G***, kibuzzard-661FBC21, F.Cu at (95.3, 51.9)
- added kibuzzard-66439A83: G***, kibuzzard-66439A83, B.Cu at (94.8, 32.7)
- added kibuzzard-66439A83: G***, kibuzzard-66439A83, B.Cu at (94.8, 82.7)
- added kibuzzard-66439ACD: G***, kibuzzard-66439ACD, B.Cu at (91.8, 76.5)
- added kibuzzard-66439ACD: G***, kibuzzard-66439ACD, B.Cu at (91.8, 26.5)
- added kibuzzard-66439AF0: G***, kibuzzard-66439AF0, B.Cu at (122.4, 63.1)
- added kibuzzard-66439AF0: G***, kibuzzard-66439AF0, B.Cu at (122.4, 113.1)
- added kibuzzard-66439B33: G***, kibuzzard-66439B33, F.Cu at (116.6, 75.9)
- added kibuzzard-66439B33: G***, kibuzzard-66439B33, F.Cu at (116.6, 25.9)
- added kibuzzard-66439B8F: G***, kibuzzard-66439B8F, F.Cu at (104.0, 60.9)
- added kibuzzard-66439B8F: G***, kibuzzard-66439B8F, F.Cu at (104.0, 110.9)
- added kibuzzard-66439C31: G***, kibuzzard-66439C31, F.Cu at (104.2, 46.5)
- added kibuzzard-66439C31: G***, kibuzzard-66439C31, F.Cu at (104.2, 96.5)
- J2 (x2): value Switching -> ExtBoard
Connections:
- net Board_0-Net-(J5-Pad1) renamed Board_0-Net-(J5-In)
- net Board_0-Net-(J6-Pad1) renamed Board_0-Net-(J6-Pin_1)
- net Board_0-Net-(J7-Pad1) renamed Board_0-Net-(J7-Pin_1)
- net Board_0-Net-(Q1-Pad3) renamed Board_0-Net-(Q1-D)
- net Board_0-Net-(Q4-Pad3) renamed Board_0-Net-(Q4-D)
- net Board_0-Net-(R14-Pad2) renamed Board_0-Net-(U10-CSB)
- net Board_0-Net-(U6-Pad5) renamed Board_0-Net-(U6-SDA)
- net Board_0-Net-(U6-Pad6) renamed Board_0-Net-(U6-SCL)
- net Board_0-unconnected-(U10-Pad5) renamed Board_0-unconnected-(U10-SDO-Pad5)
- net Board_0-unconnected-(U7-Pad1) renamed Board_0-unconnected-(U7-~{SAFEBOOT}-Pad1)
- net Board_0-unconnected-(U7-Pad14) renamed Board_0-unconnected-(U7-RESERVED-Pad14)
- net Board_0-unconnected-(U7-Pad15) renamed Board_0-unconnected-(U7-RESERVED-Pad15)
- net Board_0-unconnected-(U7-Pad16) renamed Board_0-unconnected-(U7-RESERVED-Pad16)
- net Board_0-unconnected-(U7-Pad17) renamed Board_0-unconnected-(U7-RESERVED-Pad17)
- net Board_0-unconnected-(U7-Pad3) renamed Board_0-unconnected-(U7-TIMEPULSE-Pad3)
- net Board_0-unconnected-(U7-Pad4) renamed Board_0-unconnected-(U7-EXTINT-Pad4)
- net Board_0-unconnected-(U7-Pad5) renamed Board_0-unconnected-(U7-USB_DM-Pad5)
- net Board_0-unconnected-(U7-Pad6) renamed Board_0-unconnected-(U7-USB_DP-Pad6)
- net Board_0-unconnected-(U7-Pad7) renamed Board_0-unconnected-(U7-VDD_USB-Pad7)
- net Board_1-Net-(J5-Pad1) renamed Board_1-Net-(J5-In)
- net Board_1-Net-(J6-Pad1) renamed Board_1-Net-(J6-Pin_1)
- net Board_1-Net-(J7-Pad1) renamed Board_1-Net-(J7-Pin_1)
- net Board_1-Net-(Q1-Pad3) renamed Board_1-Net-(Q1-D)
- net Board_1-Net-(Q4-Pad3) renamed Board_1-Net-(Q4-D)
- net Board_1-Net-(R14-Pad2) renamed Board_1-Net-(U10-CSB)
- net Board_1-Net-(U6-Pad5) renamed Board_1-Net-(U6-SDA)
- net Board_1-Net-(U6-Pad6) renamed Board_1-Net-(U6-SCL)
- net Board_1-unconnected-(U10-Pad5) renamed Board_1-unconnected-(U10-SDO-Pad5)
- net Board_1-unconnected-(U7-Pad1) renamed Board_1-unconnected-(U7-~{SAFEBOOT}-Pad1)
- net Board_1-unconnected-(U7-Pad14) renamed Board_1-unconnected-(U7-RESERVED-Pad14)
- net Board_1-unconnected-(U7-Pad15) renamed Board_1-unconnected-(U7-RESERVED-Pad15)
- net Board_1-unconnected-(U7-Pad16) renamed Board_1-unconnected-(U7-RESERVED-Pad16)
- net Board_1-unconnected-(U7-Pad17) renamed Board_1-unconnected-(U7-RESERVED-Pad17)
- net Board_1-unconnected-(U7-Pad3) renamed Board_1-unconnected-(U7-TIMEPULSE-Pad3)
- net Board_1-unconnected-(U7-Pad4) renamed Board_1-unconnected-(U7-EXTINT-Pad4)
- net Board_1-unconnected-(U7-Pad5) renamed Board_1-unconnected-(U7-USB_DM-Pad5)
- net Board_1-unconnected-(U7-Pad6) renamed Board_1-unconnected-(U7-USB_DP-Pad6)
- net Board_1-unconnected-(U7-Pad7) renamed Board_1-unconnected-(U7-VDD_USB-Pad7)
- J10 pad 1: Board_0-Net-(J10-Pad1) -> Board_0-Net-(J10-In)
- J10 pad 1: Board_1-Net-(J10-Pad1) -> Board_1-Net-(J10-In)
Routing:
- net Board_1-Net-(J8-Pad2): track 69.9 -> 0.00 mm
- net Board_0-Net-(J8-Pad2): track 69.9 -> 0.00 mm
- net Board_1-Net-(C1-Pad1): track 67.4 -> 0.00 mm, vias 3 -> 0
- net Board_0-Net-(C1-Pad1): track 67.4 -> 0.00 mm, vias 3 -> 0
- net Board_1-+1V8: track 48.8 -> 0.00 mm, vias 4 -> 0
- net Board_0-+1V8: track 48.8 -> 0.00 mm, vias 4 -> 0
- net Board_0-Net-(D9-A): track 0.00 -> 43.4 mm, vias 0 -> 1
- net Board_1-Net-(D9-A): track 0.00 -> 43.4 mm, vias 0 -> 1
- net Board_1-MPU_VIO_SEL: track 41.5 -> 0.00 mm, vias 2 -> 0
- net Board_0-MPU_VIO_SEL: track 41.5 -> 0.00 mm, vias 2 -> 0
- net Board_0-IO0: track 44.2 -> 3.20 mm, vias 1 -> 0
- net Board_1-IO0: track 44.2 -> 3.20 mm, vias 1 -> 0
- net Board_1-RGB: track 86.0 -> 48.9 mm
- net Board_0-RGB: track 86.0 -> 48.9 mm
- net Board_0-LORA_D1: track 0.00 -> 33.1 mm, vias 0 -> 1
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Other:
- outline, holes or cut-outs redrawn
- board text added: "+ + - OUT"
- board text added: "3V3 GND INT SCL SDA"
- board text added: "BSD-3-Clause open source hardware By @wilicw Rev. 2024.16"
- board text added: "NCKU ISP Avionics ISP32 v3.0"
- board text removed: "BSD-3-Clause open source hardware By @wilicw"
- board text removed: "NCKU ISP Avionics ISP32 v2.1"
- board text removed: "VCC GND INT SCL SDA"
